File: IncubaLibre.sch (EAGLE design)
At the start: 22 parts, among them T1 P-MOSFET

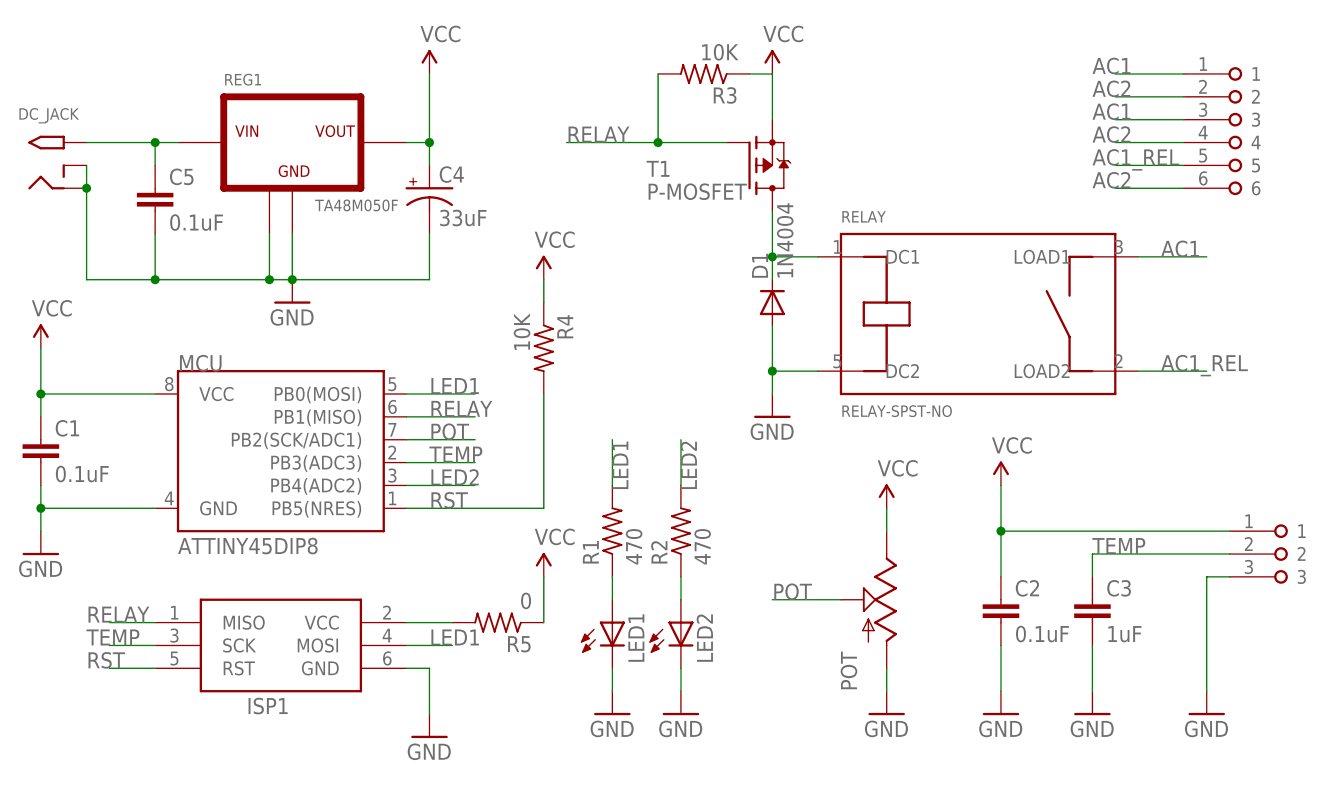
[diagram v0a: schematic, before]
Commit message: Initial buggy firmware code.
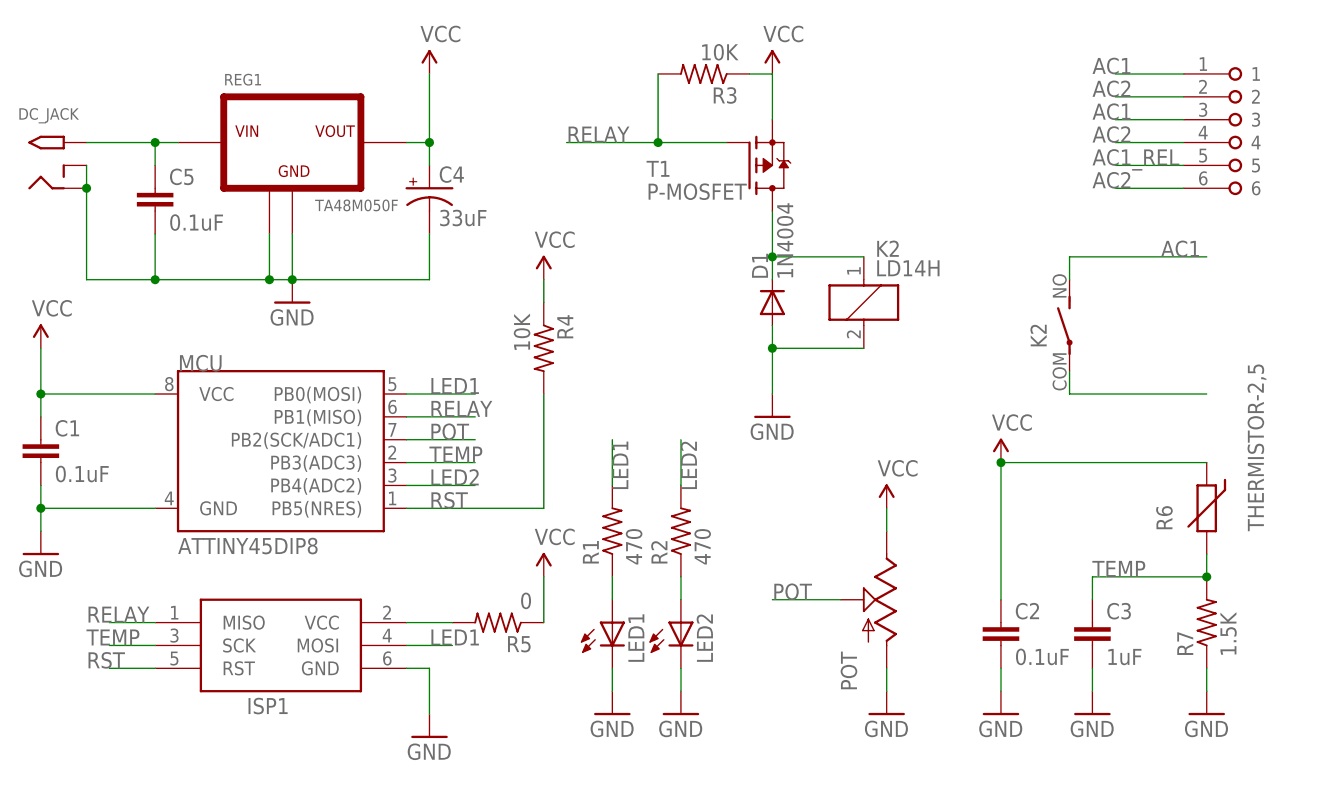
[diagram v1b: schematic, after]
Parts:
- removed RELAY: RELAY-SPST-NO, Robin:RELAY-SPST-NO
- removed SENSOR: TERMINAL-3, Robin:TERMINAL-3
- added K2: LD14H, relay:LD14H
- added R6: THERMISTOR-2,5, varistor:THERMISTOR-2,5
- added R7: 1.5K, resistor:R-US_0204/7
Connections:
- net AC1: now also K22.S; no longer RELAY.LOAD1
- net AC1_REL: now also K22.P; no longer RELAY.LOAD2
- net GND: now also K21.2, R7.1; no longer RELAY.DC2, SENSOR.3
- net T1: now also K21.1; no longer RELAY.DC1
- net TEMP: now also R6.2, R7.2; no longer SENSOR.2
- net VCC: now also R6.1; no longer SENSOR.1
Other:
- moved on the sheet: C2, C3
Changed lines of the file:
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@@
 <parts>
 <part name="MCU" library="SparkFun" deviceset="ATTINY45" device="DIP8"/>
-<part name="RELAY" library="Robin" deviceset="RELAY-SPST-NO" device=""/>
 <part name="LED1" library="adafruit" deviceset="LED" device="5MM"/>
 <part name="LED2" library="adafruit" deviceset="LED" device="5MM"/>
@@
 <part name="R4" library="resistor" deviceset="R-US_" device="0204/7" value="10K"/>
 <part name="P+7" library="SparkFun" deviceset="VCC" device=""/>
-<part name="SENSOR" library="Robin" deviceset="TERMINAL-3" device=""/>
 <part name="R5" library="resistor" deviceset="R-US_" device="0204/7" value="0"/>
+<part name="R6" library="varistor" deviceset="THERMISTOR" device="-2,5"/>
+<part name="R7" library="resistor" deviceset="R-US_" device="0204/7" value="1.5K"/>
+<part name="K2" library="relay" deviceset="LD?*" device="1" technology="4H"/>
 </parts>
 <sheets>
@@
 <instances>
 <instance part="MCU" gate="G$1" x="68.58" y="43.18"/>
-<instance part="RELAY" gate="G$1" x="144.78" y="58.42"/>
 <instance part="LED1" gate="G$1" x="104.14" y="25.4"/>
 <instance part="LED2" gate="G$1" x="111.76" y="25.4"/>
@@
 <instance part="D1" gate="1" x="121.92" y="60.96" rot="R90"/>
 <instance part="C1" gate="G$1" x="40.64" y="43.18"/>
-<instance part="C2" gate="G$1" x="147.32" y="25.4"/>
-<instance part="C3" gate="G$1" x="157.48" y="25.4"/>
+<instance part="C2" gate="G$1" x="147.32" y="22.86"/>
+<instance part="C3" gate="G$1" x="157.48" y="22.86"/>
 <instance part="GND1" gate="1" x="147.32" y="15.24"/>
 <instance part="GND2" gate="1" x="170.18" y="15.24"/>
 <instance part="GND3" gate="1" x="157.48" y="15.24"/>
 <instance part="P+1" gate="1" x="121.92" y="86.36"/>
-<instance part="P+2" gate="1" x="147.32" y="40.64"/>
+<instance part="P+2" gate="1" x="147.32" y="43.18"/>
 <instance part="P+3" gate="1" x="40.64" y="55.88"/>
 <instance part="P+4" gate="1" x="96.52" y="30.48"/>
@@
 <instance part="R4" gate="G$1" x="96.52" y="55.88" rot="R270"/>
 <instance part="P+7" gate="1" x="96.52" y="63.5"/>
-<instance part="SENSOR" gate="G$1" x="172.72" y="33.02"/>
 <instance part="R5" gate="G$1" x="91.44" y="25.4" rot="R180"/>
+<instance part="R6" gate="G$1" x="170.18" y="38.1" rot="R90"/>
+<instance part="R7" gate="G$1" x="170.18" y="25.4" rot="R90"/>
+<instance part="K2" gate="1" x="132.08" y="60.96"/>
+<instance part="K2" gate="2" x="154.94" y="58.42"/>
 </instances>
 <busses>
@@
 <segment>
 <pinref part="D1" gate="1" pin="C"/>
-<pinref part="RELAY" gate="G$1" pin="DC1"/>
-<wire x1="121.92" y1="63.5" x2="121.92" y2="66.04" width="0.1524" layer="91"/>
-<wire x1="121.92" y1="66.04" x2="127" y2="66.04" width="0.1524" layer="91"/>
-<junction x="121.92" y="66.04"/>
 <pinref part="T1" gate="G$1" pin="D"/>
 <wire x1="121.92" y1="71.12" x2="121.92" y2="66.04" width="0.1524" layer="91"/>
+<junction x="121.92" y="66.04"/>
+<wire x1="121.92" y1="66.04" x2="121.92" y2="63.5" width="0.1524" layer="91"/>
+<pinref part="K2" gate="1" pin="1"/>
+<wire x1="132.08" y1="66.04" x2="121.92" y2="66.04" width="0.1524" layer="91"/>
 </segment>
 </net>
@@
 <pinref part="C2" gate="G$1" pin="2"/>
 <pinref part="GND1" gate="1" pin="GND"/>
-<wire x1="147.32" y1="22.86" x2="147.32" y2="17.78" width="0.1524" layer="91"/>
-</segment>
-<segment>
-<pinref part="GND2" gate="1" pin="GND"/>
-<wire x1="170.18" y1="30.48" x2="170.18" y2="17.78" width="0.1524" layer="91"/>
-<pinref part="SENSOR" gate="G$1" pin="3"/>
-<wire x1="170.18" y1="30.48" x2="172.72" y2="30.48" width="0.1524" layer="91"/>
+<wire x1="147.32" y1="20.32" x2="147.32" y2="17.78" width="0.1524" layer="91"/>
 </segment>
 <segment>
 <pinref part="C3" gate="G$1" pin="2"/>
 <pinref part="GND3" gate="1" pin="GND"/>
-<wire x1="157.48" y1="22.86" x2="157.48" y2="17.78" width="0.1524" layer="91"/>
+<wire x1="157.48" y1="20.32" x2="157.48" y2="17.78" width="0.1524" layer="91"/>
 </segment>
 <segment>
 <pinref part="D1" gate="1" pin="A"/>
-<pinref part="RELAY" gate="G$1" pin="DC2"/>
-<wire x1="121.92" y1="58.42" x2="121.92" y2="53.34" width="0.1524" layer="91"/>
-<wire x1="121.92" y1="53.34" x2="127" y2="53.34" width="0.1524" layer="91"/>
-<junction x="121.92" y="53.34"/>
 <pinref part="GND4" gate="1" pin="GND"/>
-<wire x1="121.92" y1="53.34" x2="121.92" y2="50.8" width="0.1524" layer="91"/>
+<wire x1="121.92" y1="58.42" x2="121.92" y2="55.88" width="0.1524" layer="91"/>
+<junction x="121.92" y="55.88"/>
+<wire x1="121.92" y1="55.88" x2="121.92" y2="50.8" width="0.1524" layer="91"/>
+<pinref part="K2" gate="1" pin="2"/>
+<wire x1="132.08" y1="55.88" x2="121.92" y2="55.88" width="0.1524" layer="91"/>
 </segment>
 <segment>
@@
 <wire x1="111.76" y1="20.32" x2="111.76" y2="17.78" width="0.1524" layer="91"/>
 </segment>
+<segment>
+<pinref part="GND2" gate="1" pin="GND"/>
+<pinref part="R7" gate="G$1" pin="1"/>
+<wire x1="170.18" y1="20.32" x2="170.18" y2="17.78" width="0.1524" layer="91"/>
+</segment>
 </net>
 <net name="RELAY" class="0">
@@
 <segment>
 <pinref part="C2" gate="G$1" pin="1"/>
-<wire x1="147.32" y1="30.48" x2="147.32" y2="35.56" width="0.1524" layer="91"/>
-<wire x1="147.32" y1="35.56" x2="172.72" y2="35.56" width="0.1524" layer="91"/>
-<junction x="147.32" y="35.56"/>
 <pinref part="P+2" gate="1" pin="VCC"/>
-<wire x1="147.32" y1="40.64" x2="147.32" y2="35.56" width="0.1524" layer="91"/>
-<pinref part="SENSOR" gate="G$1" pin="1"/>
+<wire x1="147.32" y1="43.18" x2="147.32" y2="27.94" width="0.1524" layer="91"/>
+<junction x="147.32" y="43.18"/>
+<pinref part="R6" gate="G$1" pin="1"/>
+<wire x1="170.18" y1="43.18" x2="147.32" y2="43.18" width="0.1524" layer="91"/>
 </segment>
 <segment>
@@
 <net name="AC1" class="0">
 <segment>
-<pinref part="RELAY" gate="G$1" pin="LOAD1"/>
-<wire x1="162.56" y1="66.04" x2="170.18" y2="66.04" width="0.1524" layer="91"/>
 <label x="165.1" y="66.04" size="1.778" layer="95"/>
+<wire x1="154.94" y1="63.5" x2="154.94" y2="66.04" width="0.1524" layer="91"/>
+<wire x1="154.94" y1="66.04" x2="170.18" y2="66.04" width="0.1524" layer="91"/>
+<pinref part="K2" gate="2" pin="S"/>
 </segment>
 <segment>
@@
 <net name="AC1_REL" class="0">
 <segment>
-<pinref part="RELAY" gate="G$1" pin="LOAD2"/>
-<wire x1="162.56" y1="53.34" x2="170.18" y2="53.34" width="0.1524" layer="91"/>
-<label x="165.1" y="53.34" size="1.778" layer="95"/>
-</segment>
-<segment>
 <pinref part="AC" gate="G$1" pin="5"/>
 <wire x1="167.64" y1="76.2" x2="160.02" y2="76.2" width="0.1524" layer="91"/>
 <label x="157.48" y="76.2" size="1.778" layer="95"/>
+</segment>
+<segment>
+<wire x1="154.94" y1="50.8" x2="170.18" y2="50.8" width="0.1524" layer="91"/>
+<wire x1="154.94" y1="53.34" x2="154.94" y2="50.8" width="0.1524" layer="91"/>
+<pinref part="K2" gate="2" pin="P"/>
 </segment>
 </net>
@@
 <segment>
 <pinref part="C3" gate="G$1" pin="1"/>
-<wire x1="172.72" y1="33.02" x2="157.48" y2="33.02" width="0.1524" layer="91"/>
-<wire x1="157.48" y1="33.02" x2="157.48" y2="30.48" width="0.1524" layer="91"/>
-<label x="157.48" y="33.02" size="1.778" layer="95"/>
-<pinref part="SENSOR" gate="G$1" pin="2"/>
-</segment>
-<segment>
+<wire x1="157.48" y1="30.48" x2="157.48" y2="27.94" width="0.1524" layer="91"/>
+<label x="157.48" y="30.48" size="1.778" layer="95"/>
+<pinref part="R7" gate="G$1" pin="2"/>
+<junction x="170.18" y="30.48"/>
+<pinref part="R6" gate="G$1" pin="2"/>
+<wire x1="170.18" y1="33.02" x2="170.18" y2="30.48" width="0.1524" layer="91"/>
+<wire x1="157.48" y1="30.48" x2="170.18" y2="30.48" width="0.1524" layer="91"/>
+</segment>
+<segment>
